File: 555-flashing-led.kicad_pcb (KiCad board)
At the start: 2 copper layers, 66.8 x 98.6 mm, 9 parts, among them U1 7555

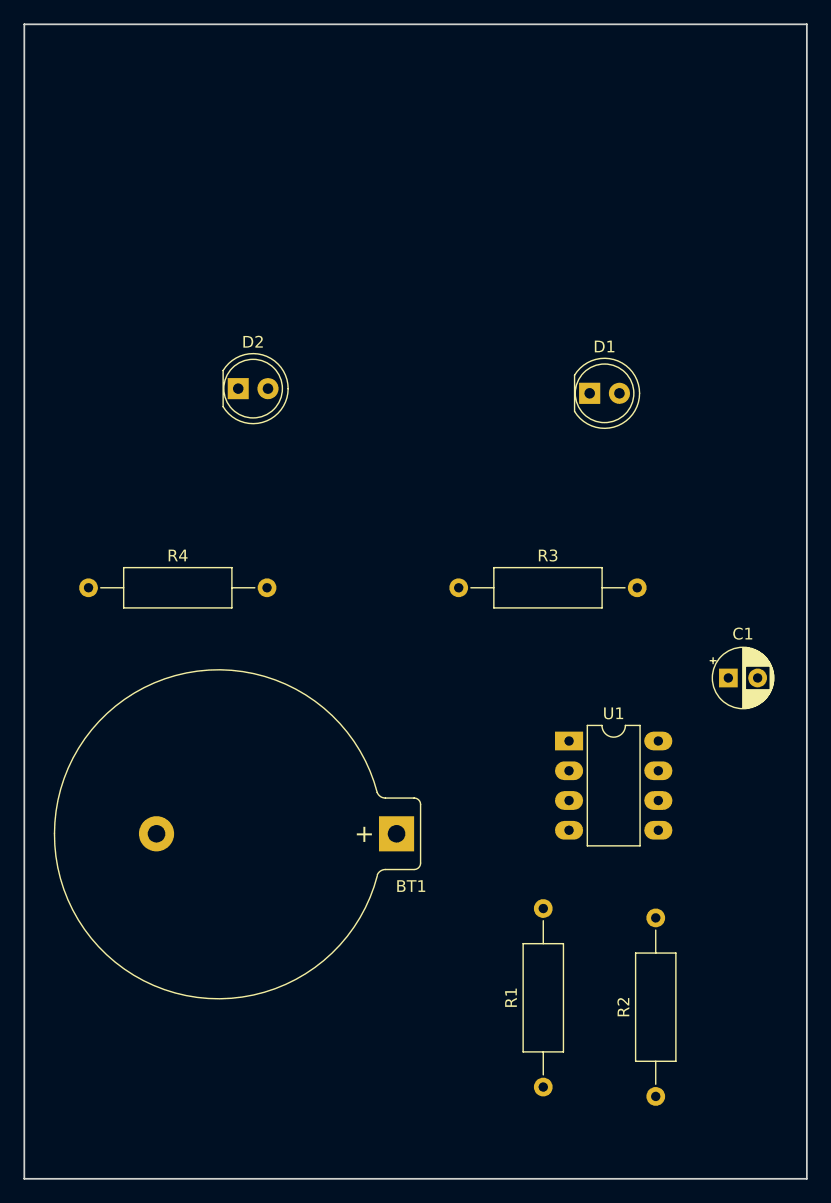
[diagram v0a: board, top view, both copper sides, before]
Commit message: finalize pcb
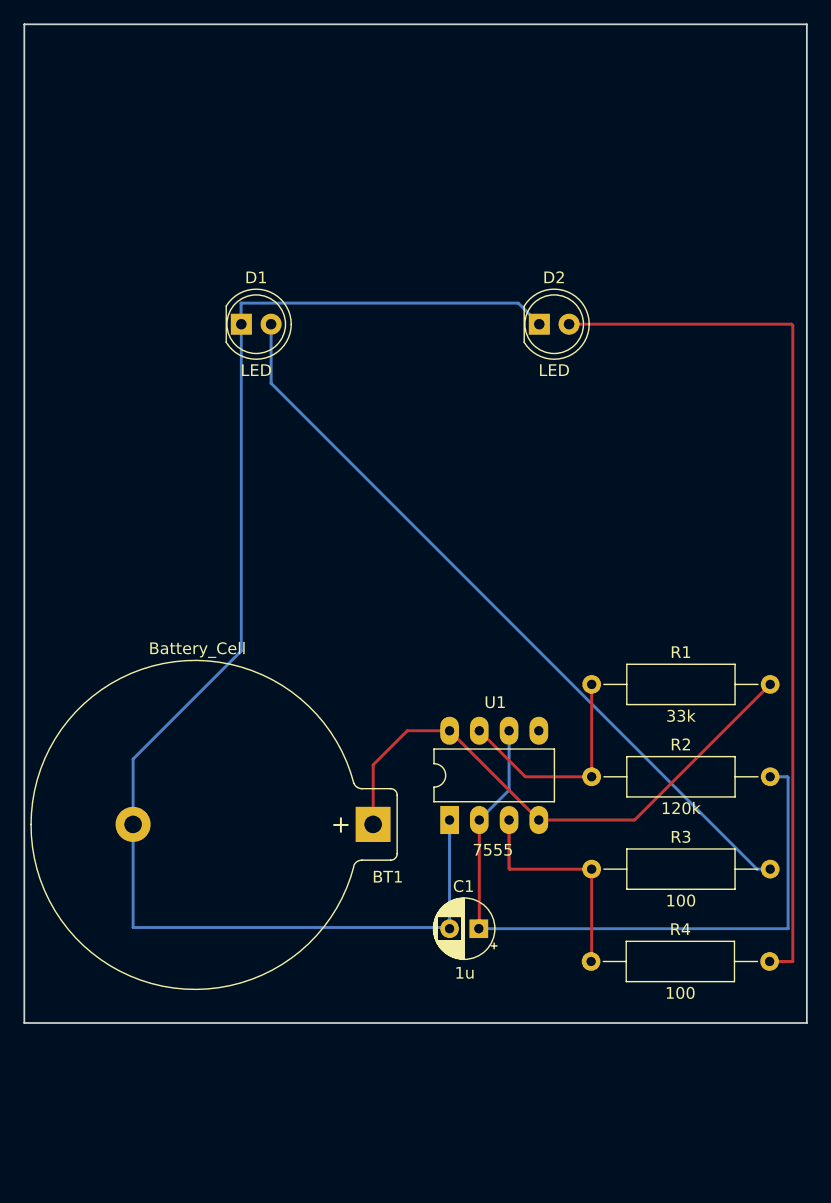
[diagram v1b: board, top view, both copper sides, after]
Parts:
- R3, R4: value 1k -> 100
- moved R4 53.5 mm to (114.0, 110.0)
- moved R1 34.6 mm to (114.0, 86.3), turned to 0 degrees
- moved D1 30.3 mm to (84.1, 55.6)
- moved C1 30.2 mm to (104.4, 107.2), turned to 180 degrees
- moved R2 27.8 mm to (114.0, 94.2), turned to 0 degrees
- moved R3 26.6 mm to (114.0, 102.1)
- moved D2 26.3 mm to (109.6, 55.6)
- moved U1 12.2 mm to (101.9, 97.9), turned to 90 degrees
- moved BT1 2.15 mm to (95.4, 98.3)
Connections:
- BT1 pad 1: GNDREF -> +3V0
- BT1 pad 2: +3V0 -> GNDREF
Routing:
- net GNDREF: track 0.00 -> 119.7 mm
- net Net-(D2-A): track 0.00 -> 75.4 mm
- net Net-(D1-A): track 0.00 -> 64.8 mm
- net Net-(U1-THRESHOLD): track 0.00 -> 58.8 mm
- net +3V0: track 0.00 -> 48.1 mm
- net Net-(U1-OUTPUT): track 0.00 -> 19.1 mm
- net Net-(U1-DISCHARGE): track 0.00 -> 19.1 mm
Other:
- board size 66.8 x 98.6 mm -> 66.8 x 85.3 mm
